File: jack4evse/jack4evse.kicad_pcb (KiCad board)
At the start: 2 copper layers, 24.8 x 87.1 mm, 10 parts, among them J1 Conn_02x08_Odd_Even, J2 Conn_01x04, J3 Conn_01x04, J4 Conn_02x08_Odd_Even, J5 Conn_01x04, J6 Conn_01x04

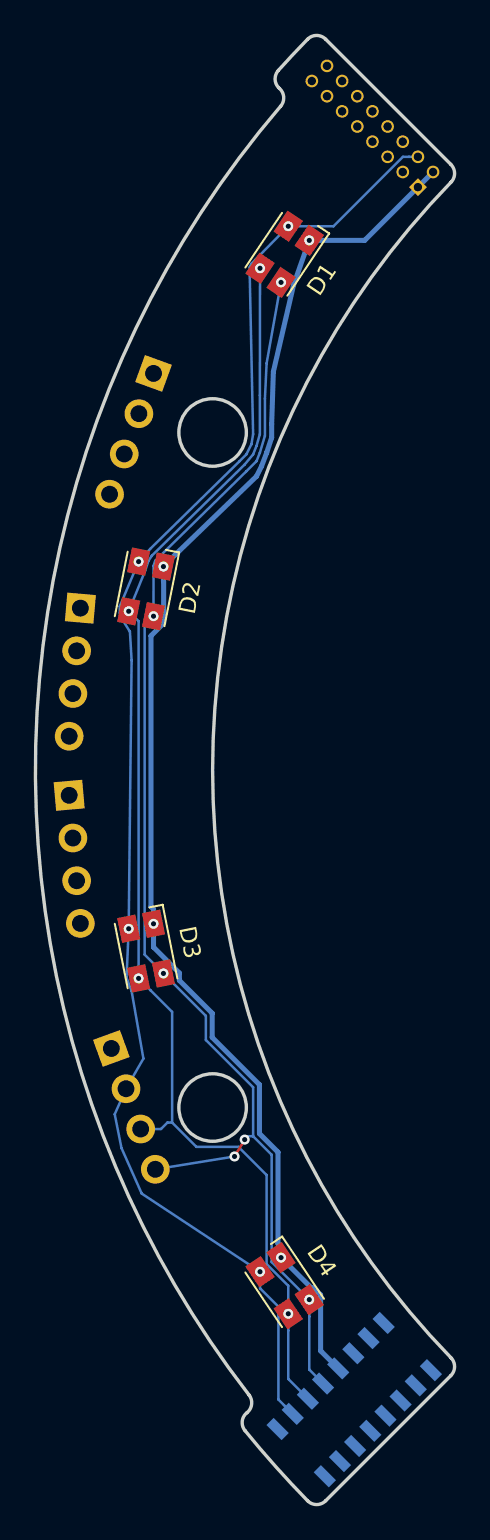
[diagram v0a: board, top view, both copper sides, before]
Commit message: jack/pcb: Done routing
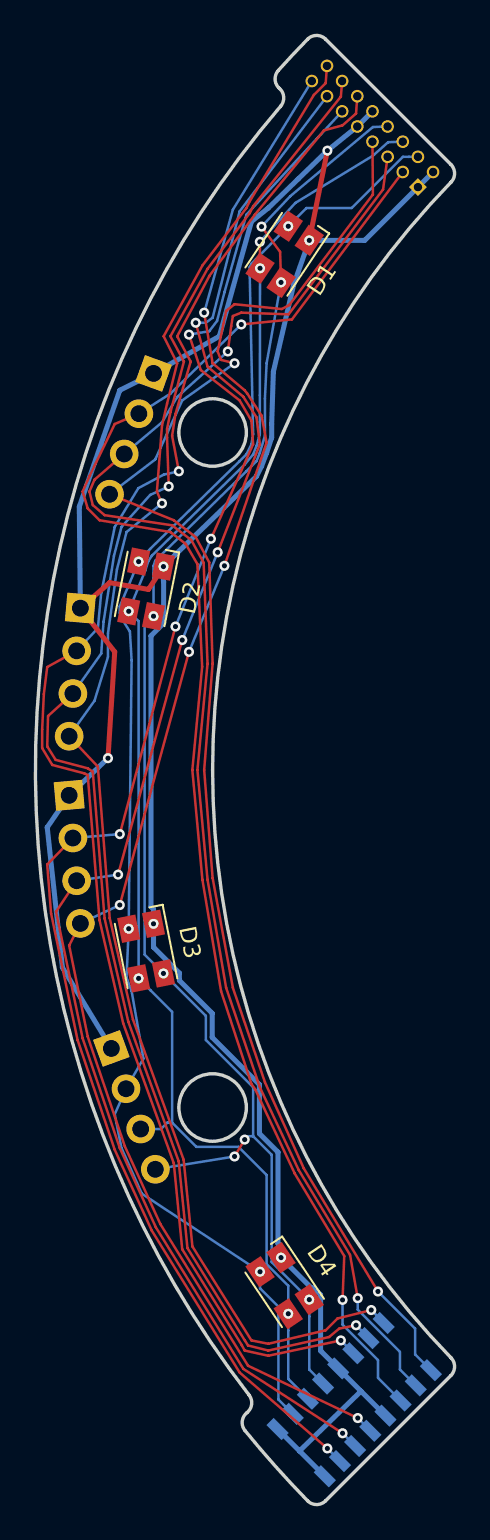
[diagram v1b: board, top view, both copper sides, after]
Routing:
- net /R1: track 0.00 -> 94.8 mm, vias 0 -> 5
- net /G1: track 0.00 -> 93.9 mm, vias 0 -> 5
- net /R2: track 0.00 -> 92.8 mm, vias 0 -> 2
- net /B1: track 0.00 -> 92.6 mm, vias 0 -> 5
- net /G2: track 0.00 -> 92.5 mm, vias 0 -> 2
- net /B2: track 0.00 -> 91.5 mm, vias 0 -> 2
- net +5V: track 83.7 -> 174.2 mm, vias 4 -> 6
- net /R3: track 0.00 -> 89.7 mm, vias 0 -> 2
- net /G3: track 0.00 -> 89.3 mm, vias 0 -> 2
- net /B3: track 0.00 -> 89.0 mm, vias 0 -> 2
- net /B0: track 79.0 -> 92.4 mm, vias 6 -> 7
- net /G0: track 77.7 -> 89.8 mm, vias 4 -> 5
